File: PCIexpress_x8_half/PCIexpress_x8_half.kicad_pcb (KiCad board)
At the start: 4 copper layers, 167.7 x 111.2 mm, 34 parts, among them J1 PCIexpress_bracket, J2 PCIexpress_x8

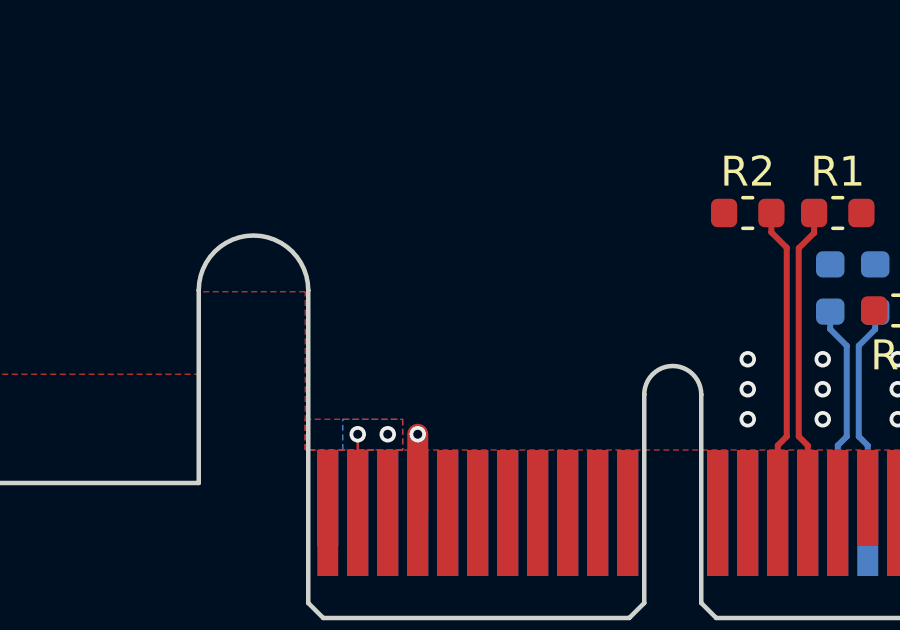
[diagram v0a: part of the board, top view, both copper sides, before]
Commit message: KiCad 6 update
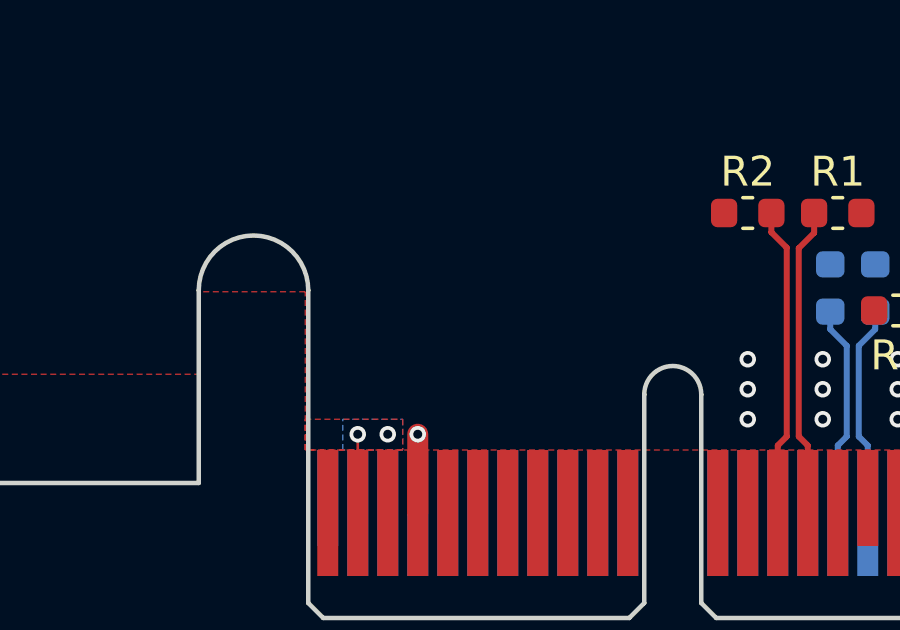
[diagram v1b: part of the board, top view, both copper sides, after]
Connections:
- net /~PERST renamed /~{PERST}
- net /~PRSNT1 renamed /~{PRSNT1}
- net /~PRSNT2x1 renamed /~{PRSNT2x1}
- net /~PRSNT2x4 renamed /~{PRSNT2x4}
- net /~PRSNT2x8 renamed /~{PRSNT2x8}
- net /~TRST renamed /~{TRST}
- net /~WAKE renamed /~{WAKE}
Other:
- net class Default removed
- net class Diff-100-PCIe removed
- net class JLC2313-100d-3.5 removed
- net class JLC2313-100d-4 removed
- net class JLC7628-100d-8 removed
